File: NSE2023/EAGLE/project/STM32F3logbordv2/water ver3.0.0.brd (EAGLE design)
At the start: 30 x 30 mm, 11 parts

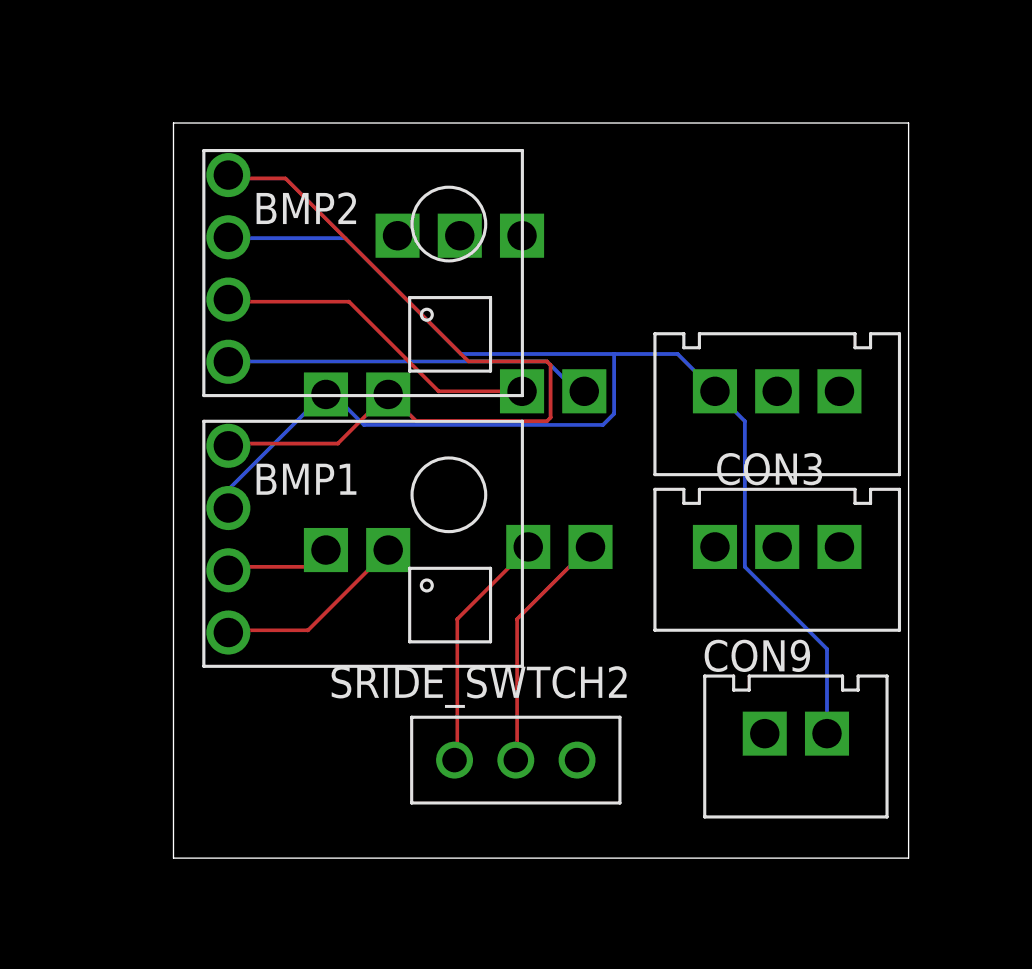
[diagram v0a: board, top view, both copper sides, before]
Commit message: create final board
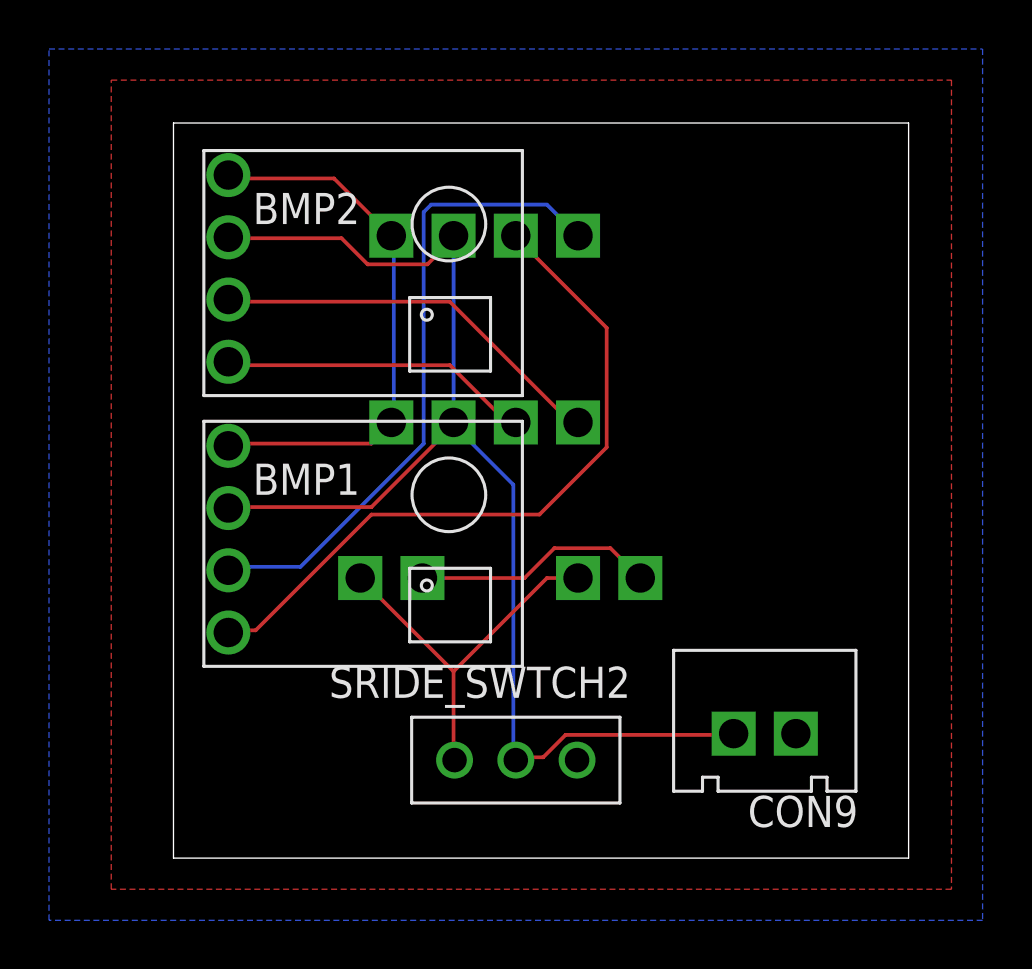
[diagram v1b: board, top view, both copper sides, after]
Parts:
- removed CON3, CON5, CON7: (no value), XR Connector:3PIN
- removed CON4, CON6: (no value), XR Connector:2PIN
- added SIGNAL, SIGNAL1: (no value), XR Connector:4PIN_SIDE
- moved CON2 7.96 mm to (17.8, 11.4)
- moved CON1 1.81 mm to (8.89, 11.4)
- moved CON9 1.27 mm to (24.1, 5.08), turned to 180 degrees
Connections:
- removed net +5V: CON7.P$2
- removed net N$3: CON6.P$2, SRIDE_SWTCH2.L
- removed net N$4: CON6.P$1, SRIDE_SWTCH2.LR
- removed net PWM: CON7.P$3
- new net FPRAW: CON1.P$1, CON2.P$1
- new net SWITCH: CON1.P$2, CON2.P$2, SRIDE_SWTCH2.L
- net +3V3: now also SIGNAL.P$3, SIGNAL1.P$3; no longer CON4.P$1
- net GND: now also SIGNAL.P$4, SIGNAL1.P$4, SRIDE_SWTCH2.LR; no longer CON4.P$2, CON7.P$1
- net SCL0: now also SIGNAL.P$1; no longer CON1.P$2
- net SCL1: now also SIGNAL1.P$1; no longer CON2.P$2
- net SDA0: now also SIGNAL.P$2; no longer CON1.P$1
- net SDA1: now also SIGNAL1.P$2; no longer CON2.P$1
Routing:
- net SCL0: track 4.36 -> 26.6 mm
- net SDA0: track 7.94 -> 28.7 mm
- net SWITCH: track 0.00 -> 15.7 mm
- net +3V3: track 33.1 -> 22.5 mm
- net N$4: track 9.97 -> 0.00 mm
- net N$3: track 9.95 -> 0.00 mm
- net FPRAW: track 0.00 -> 9.90 mm
- net GND: track 59.6 -> 52.7 mm
- net SCL1: track 13.6 -> 16.4 mm
- net SDA1: track 15.0 -> 12.8 mm
- added copper zone on layer 1, net GND
- added copper zone on layer 16, net GND
